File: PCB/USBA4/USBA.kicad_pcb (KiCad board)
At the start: 2 copper layers, 70 x 70 mm, 23 parts, among them J1 USB_A, J2 Shelly, U2 ESP32-S3-MINI-1, U5 MD8942, U6 SHT40

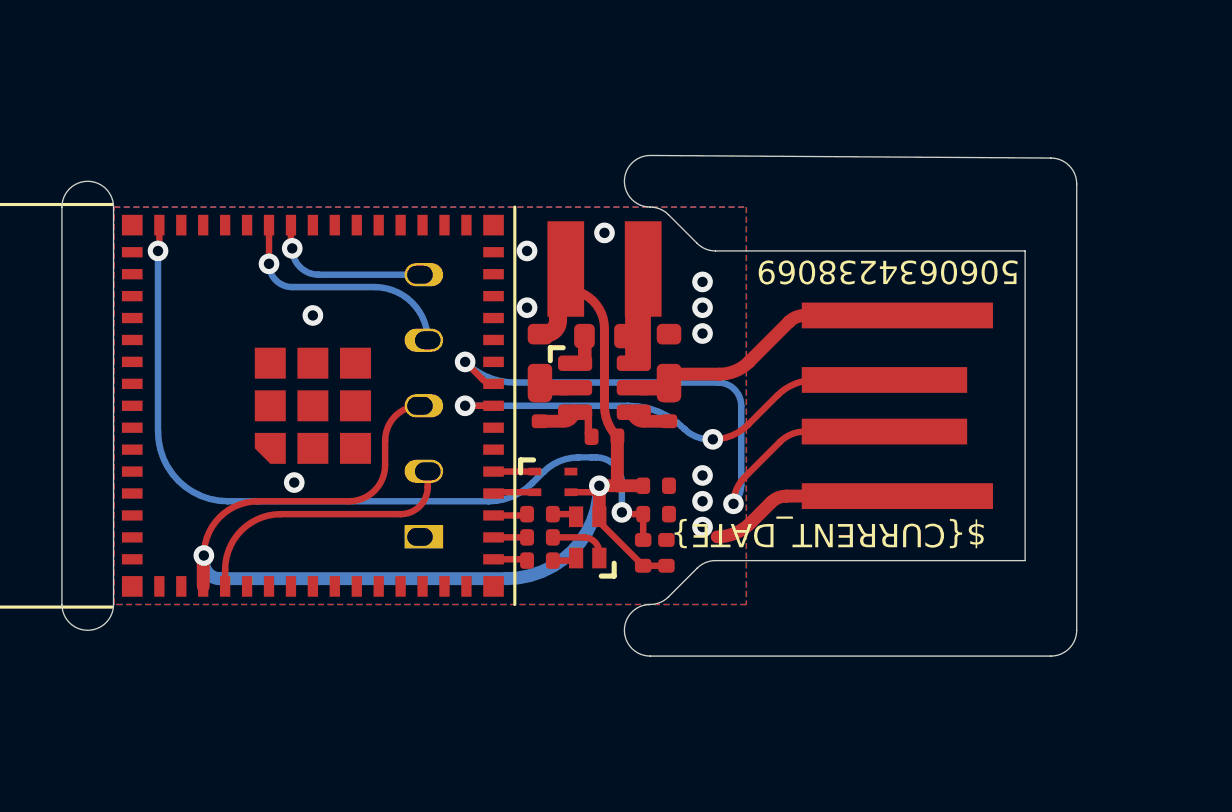
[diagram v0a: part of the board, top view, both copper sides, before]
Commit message: SMaller
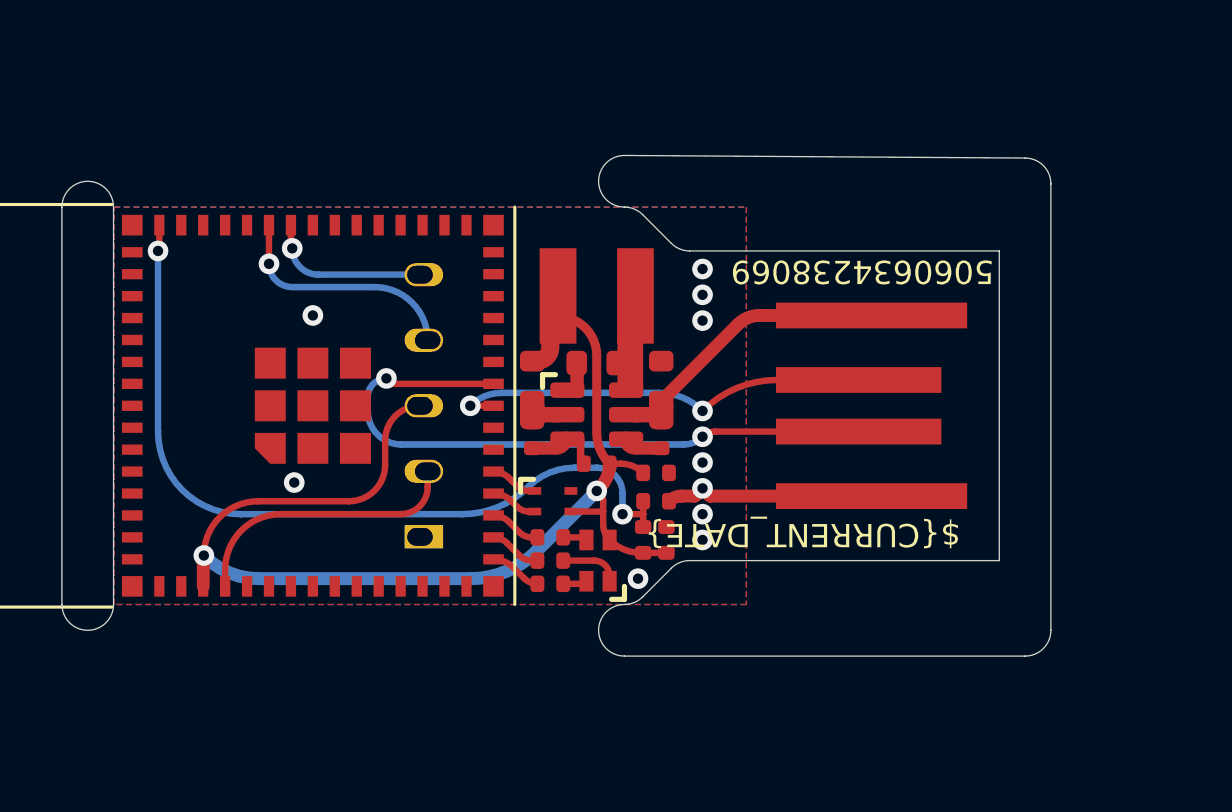
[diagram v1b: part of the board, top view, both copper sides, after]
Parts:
- moved C6 1.09 mm to (106.9, 98.3)
- moved C7 1.09 mm to (101.9, 98.3)
- moved C8 1.09 mm to (104.4, 97.6)
- moved L2 1.09 mm to (104.4, 95.0)
- moved R9 1.09 mm to (104.4, 101.5)
- moved U5 1.09 mm to (104.4, 99.6)
- moved R10 1.09 mm to (101.9, 100.4)
- moved R11 1.09 mm to (106.9, 100.4)
- moved J1 1.00 mm to (120.0, 99.3)
- moved R5 0.98 mm to (102.6, 106.2)
- moved R7 0.98 mm to (102.6, 104.4)
- moved D2 0.98 mm to (104.5, 105.3)
- moved R4 0.98 mm to (102.6, 105.3)
- moved U6 0.75 mm to (102.7, 103.0)
- moved C1 0.50 mm to (106.7, 101.9)
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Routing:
- net +3.3V: track 40.3 -> 37.9 mm
- net D+: track 23.9 -> 25.7 mm
- net D-: track 15.7 -> 16.6 mm
- net G: track 1.25 -> 2.01 mm
- net B: track 1.25 -> 1.98 mm
- net R: track 1.30 -> 2.01 mm
- net GND: track 7.51 -> 8.15 mm, vias 11 -> 10
